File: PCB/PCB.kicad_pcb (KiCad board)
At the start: 2 copper layers, 120.6 x 100.3 mm, 27 parts, among them J1 Conn_01x04_Female, J2 Conn_01x04_Female, J3 Conn_01x04_Female, J4 Conn_01x04_Female, J5 MiniMicroJst2.0Ph3Pin, J6 Conn_01x02_Female, J7 Conn_01x02_Female, U1 ESP01

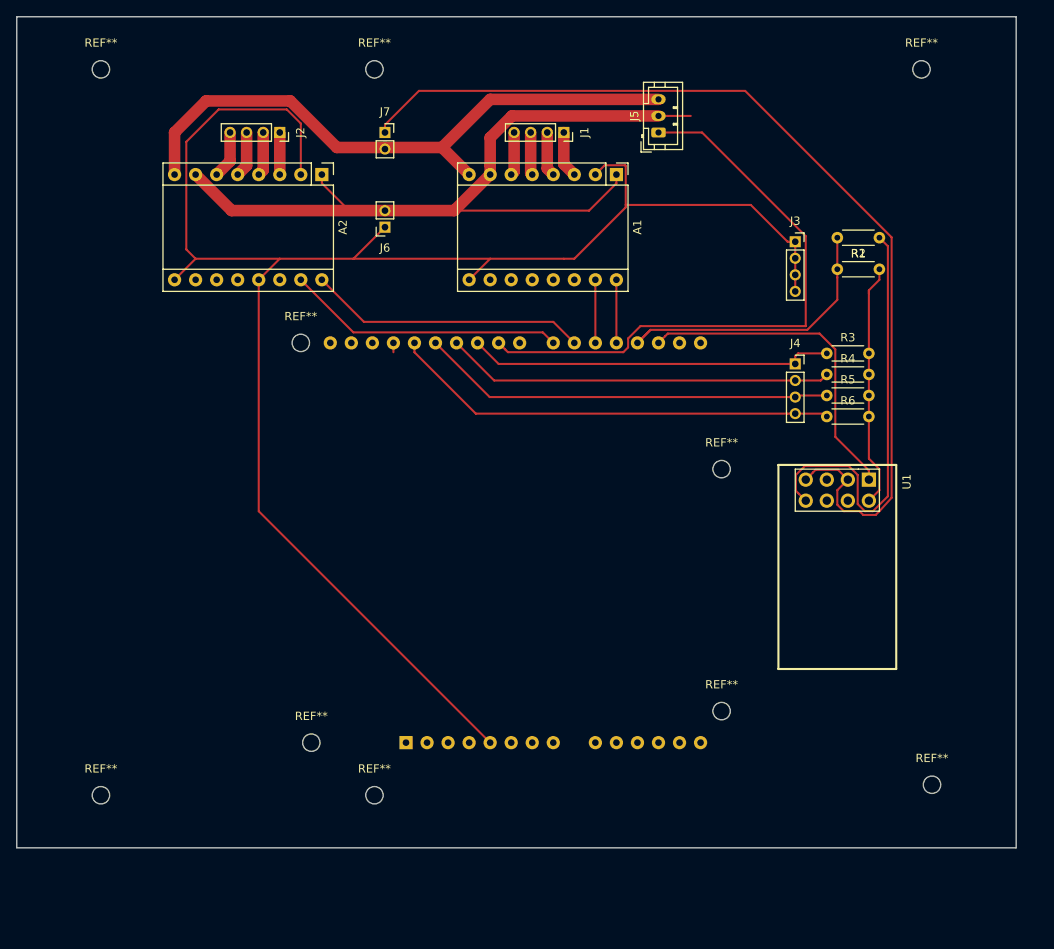
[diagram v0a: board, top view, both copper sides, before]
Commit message: m
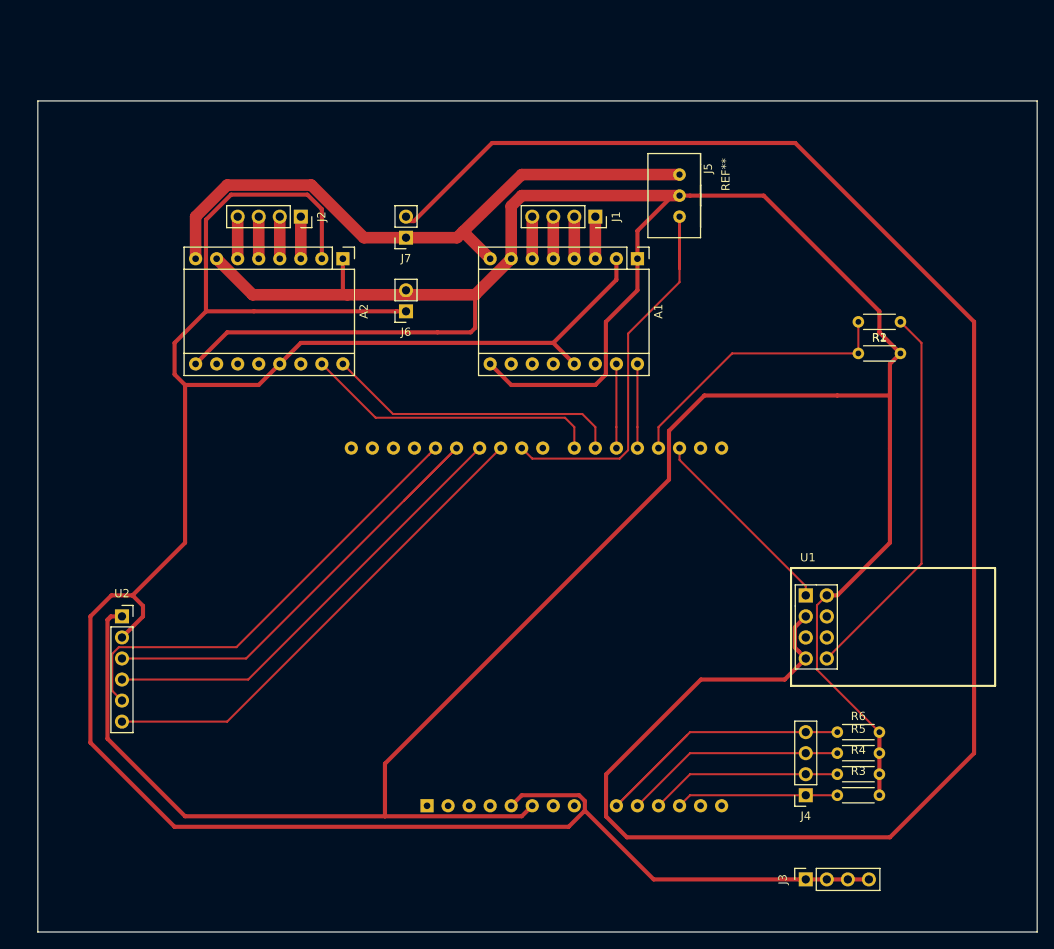
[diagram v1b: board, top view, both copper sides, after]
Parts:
- removed REF** (x10): MountingHole_2.1mm, MountingHole:MountingHole_2.1mm
- added U2: MicroSDCardModule, Connector_PinSocket_2.54mm:PinSocket_1x06_P2.54mm_Vertical, F.Cu at (120.7, 85.1)
- J1, J2, J3, J4: footprint Connector_PinSocket_2.00mm:PinSocket_1x04_P2.00mm_Vertical -> Connector_PinSocket_2.54mm:PinSocket_1x04_P2.54mm_Vertical
- J5: footprint Connector_JST:JST_PH_B3B-PH-K_1x03_P2.00mm_Vertical -> PCB:mini micro jst 2.02ph 3pin
- J6, J7: footprint Connector_PinSocket_2.00mm:PinSocket_1x02_P2.00mm_Vertical -> Connector_PinSocket_2.54mm:PinSocket_1x02_P2.54mm_Vertical
- R1: value 1k -> R
- R2: value 2k -> R
- R3, R4, R5, R6: value 4,7k -> 4.7k
- moved J3 77.0 mm to (203.2, 116.8), turned to 90 degrees
- moved R3 53.4 mm to (207.0, 106.7)
- moved J4 52.1 mm to (203.2, 106.7), turned to 180 degrees
- moved R4 48.3 mm to (207.0, 104.1)
- moved R5 43.2 mm to (207.0, 101.6)
- moved R6 38.1 mm to (207.0, 99.1)
- moved U1 15.9 mm to (203.2, 82.5), turned to 0 degrees
- moved J7 13.0 mm to (154.9, 39.4), turned to 180 degrees
- moved J5 10.9 mm to (194.3, 33.0)
- moved J1 10.9 mm to (177.8, 36.8)
- moved R2 10.5 mm to (209.6, 53.3)
- moved J2 10.5 mm to (142.2, 36.8)
- moved R1 10.5 mm to (214.6, 49.5)
- moved A1 10.5 mm to (182.9, 41.9)
- moved A2 10.5 mm to (147.3, 41.9)
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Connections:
- A1 pad 9: VCC -> GND
- A2 pad 9: VCC -> GND
- A3 pad 29: GND -> Net-(A3-Pad29)
- A3 pad 6: Net-(A3-Pad6) -> GND
- J4 pad 1: Net-(A3-Pad25) -> Net-(A3-Pad12)
- J4 pad 2: Net-(A3-Pad26) -> Net-(A3-Pad11)
- J4 pad 3: Net-(A3-Pad27) -> Net-(A3-Pad10)
- J4 pad 4: Net-(A3-Pad28) -> Net-(A3-Pad9)
- J7 pad 1: +3V3 -> +12V
- J7 pad 2: +12V -> +3V3
- R3 pad 1: Net-(A3-Pad25) -> Net-(A3-Pad12)
- R4 pad 1: Net-(A3-Pad26) -> Net-(A3-Pad11)
- R5 pad 1: Net-(A3-Pad27) -> Net-(A3-Pad10)
- R6 pad 1: Net-(A3-Pad28) -> Net-(A3-Pad9)
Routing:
- net GND: track 140.4 -> 422.3 mm
- net +3V3: track 120.1 -> 224.3 mm
- net VCC: track 212.5 -> 301.5 mm
- net Net-(A3-Pad9): track 0.00 -> 42.4 mm
- net Net-(A3-Pad10): track 0.00 -> 26.8 mm
- net Net-(A3-Pad11): track 0.00 -> 23.2 mm
- net Net-(A3-Pad24): track 73.3 -> 50.9 mm
- net Net-(A3-Pad12): track 0.00 -> 19.6 mm
- net Net-(A3-Pad17): track 40.0 -> 24.1 mm
- net Net-(A3-Pad25): track 44.3 -> 59.4 mm
- net Net-(A3-Pad27): track 50.0 -> 59.9 mm
- net Net-(A3-Pad26): track 46.9 -> 54.8 mm
- net Net-(R1-Pad1): track 51.9 -> 46.4 mm
- net Net-(A2-Pad16): track 33.6 -> 36.2 mm
- net Net-(A2-Pad15): track 33.6 -> 36.2 mm
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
